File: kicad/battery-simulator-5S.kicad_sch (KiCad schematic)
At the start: 58 parts, among them J1 Conn_power_brd, J2 Conn_ctrl_brd, J7 Barrel_Jack, Q1 2N3904, Q2 NDP6020P, Q3 2SD2390, U1 LM324, U3 TL431LP, U4 LM317_TO-220

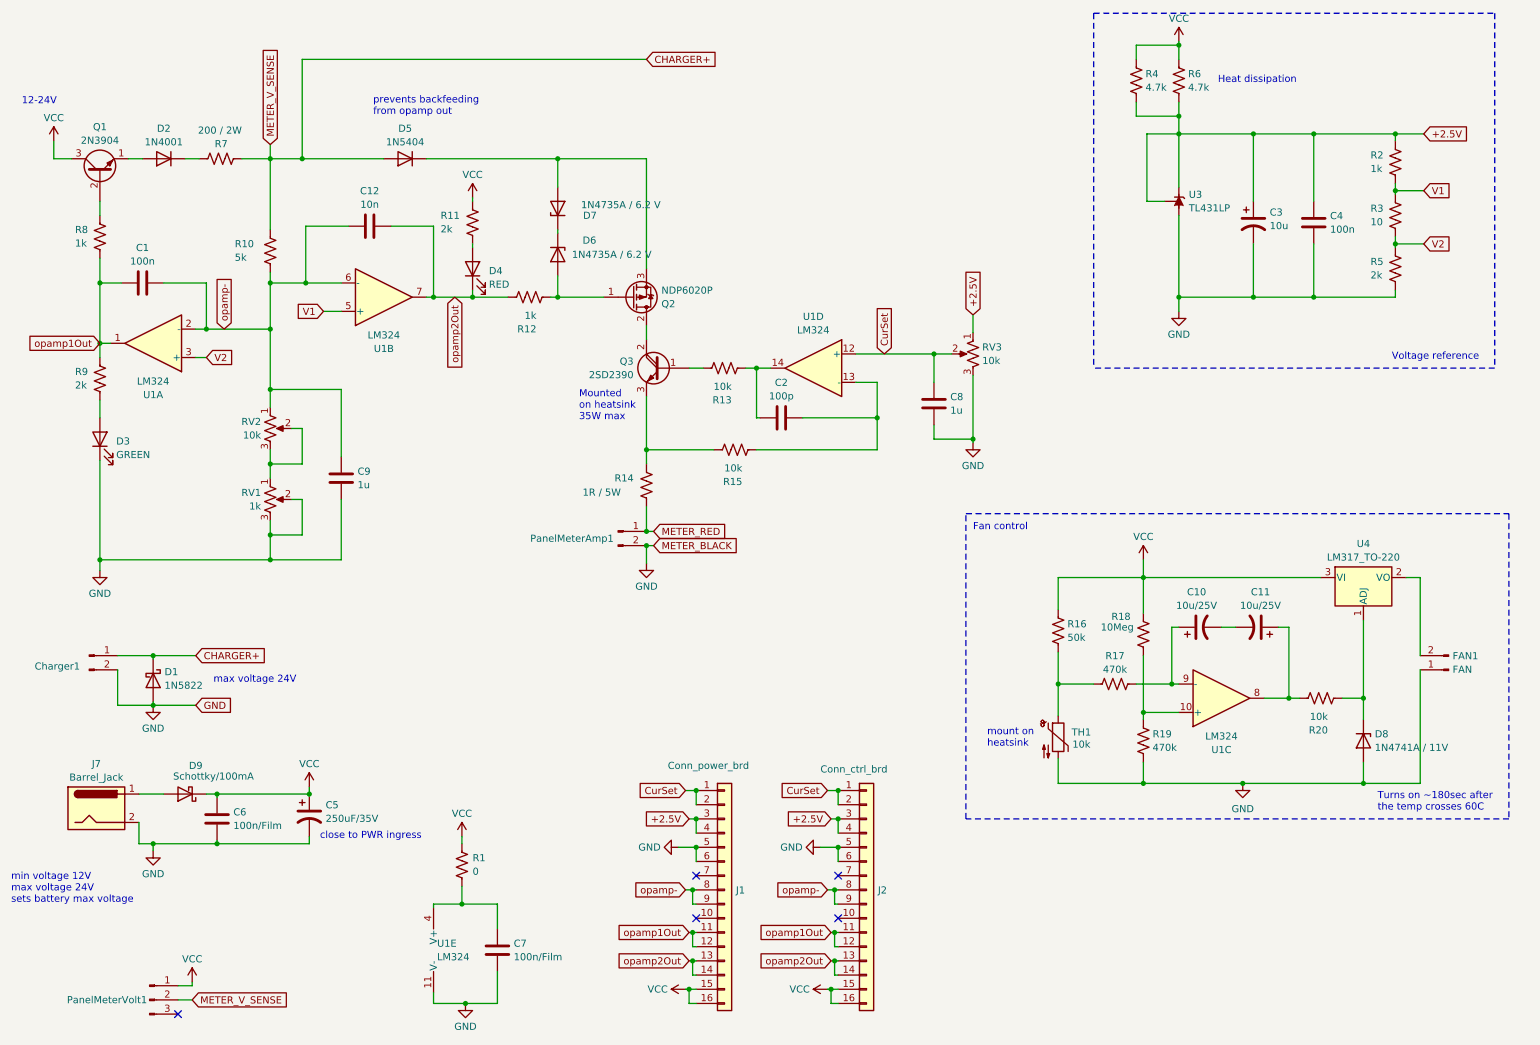
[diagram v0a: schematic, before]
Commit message: More ideas
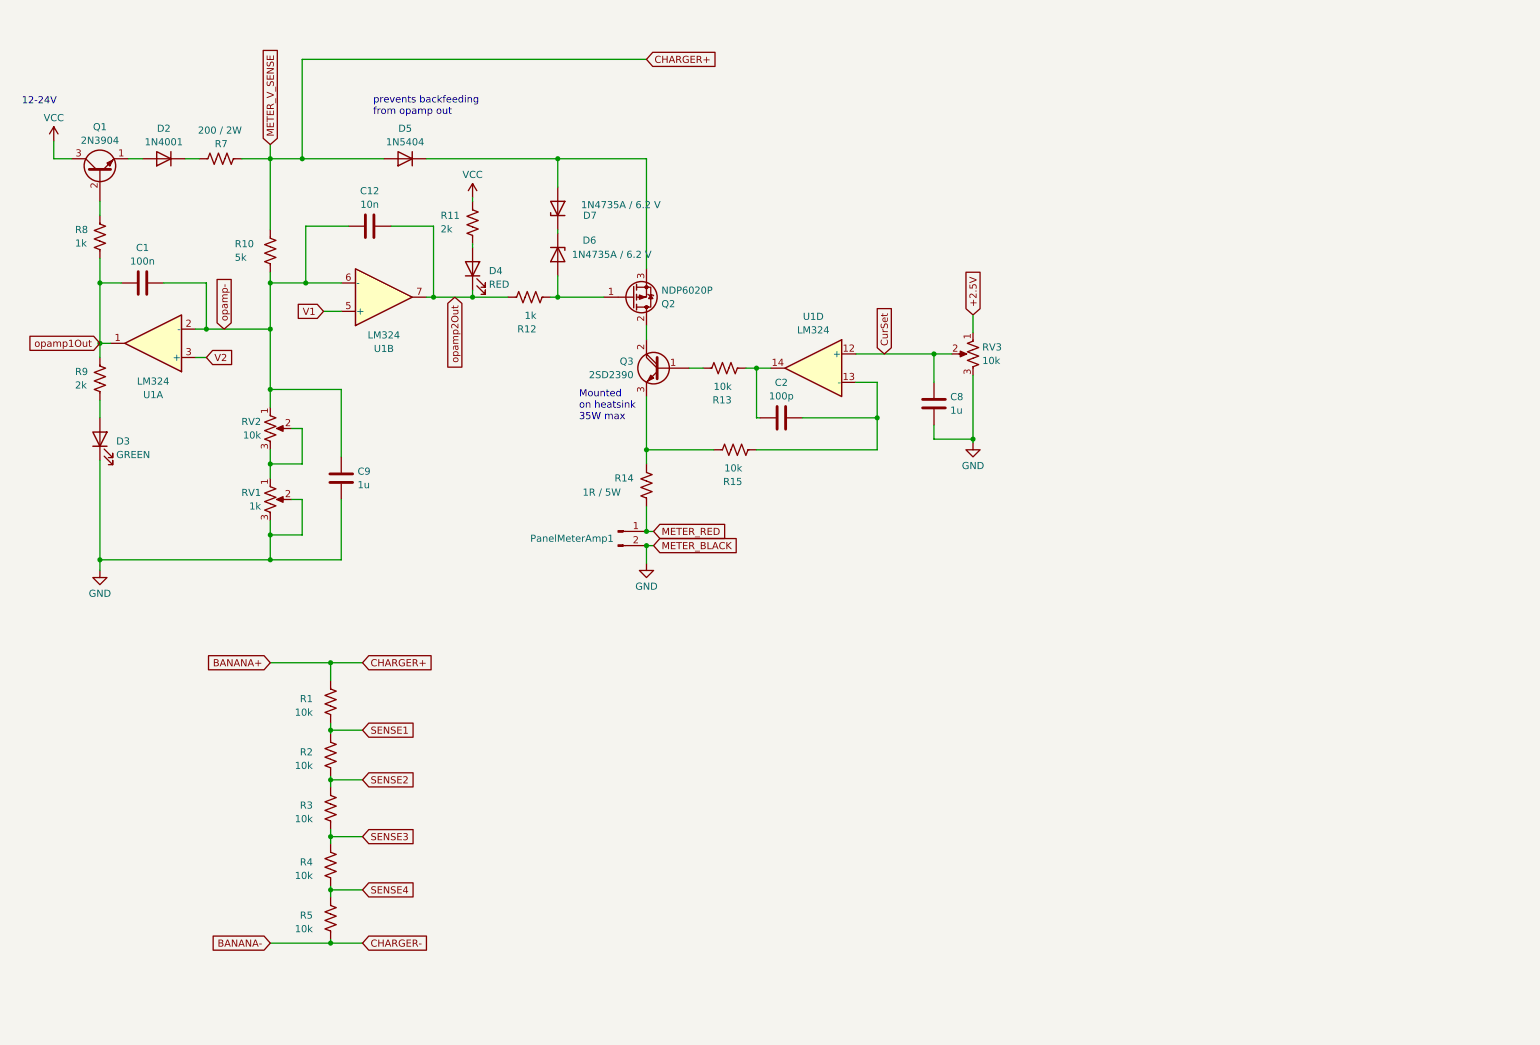
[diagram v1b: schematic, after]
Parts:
- removed C10, C11: 10u/25V, Capacitor_THT:CP_Radial_D5.0mm_P2.50mm, symbol Device:C_Polarized_US
- removed C3: 10u, Capacitor_THT:CP_Radial_D5.0mm_P2.50mm, symbol Device:C_Polarized_US
- removed C4: 100n, Capacitor_SMD:C_1206_3216Metric, symbol Device:C
- removed C5: 250uF/35V, Capacitor_THT:CP_Radial_D14.0mm_P5.00mm, symbol Device:C_Polarized_US
- removed C6, C7: 100n/Film, Capacitor_SMD:C_1206_3216Metric, symbol Device:C
- removed Charger1: Charger, Connector_Phoenix_MC_HighVoltage:PhoenixContact_MCV_1,5_2-G-5.08_1x02_P5.08mm_Vertical, symbol Connector:Conn_01x02_Pin
- removed D1: 1N5822, Diode_THT:D_DO-201AD_P5.08mm_Vertical_AnodeUp, symbol Diode:1N5822
- removed D8: 1N4741A / 11V, Diode_THT:D_DO-35_SOD27_P5.08mm_Vertical_KathodeUp, symbol Device:D_Zener
- removed D9: Schottky/100mA, Diode_SMD:D_SMA, symbol Device:D_Schottky
- removed FAN1: FAN, Connector_PinHeader_2.54mm:PinHeader_1x03_P2.54mm_Vertical, symbol Connector:Conn_01x02_Pin
- removed J1: Conn_power_brd, Connector_PinSocket_2.54mm:PinSocket_1x16_P2.54mm_Vertical, symbol Connector_Generic:Conn_01x16
- removed J2: Conn_ctrl_brd, Connector_PinHeader_2.54mm:PinHeader_1x16_P2.54mm_Horizontal, symbol Connector_Generic:Conn_01x16
- removed J7: Barrel_Jack, Connector_BarrelJack:BarrelJack_Horizontal, symbol Connector:Barrel_Jack
- removed PanelMeterVolt1: Panel Meter Volt, Connector_JST:JST_XH_B3B-XH-A_1x03_P2.50mm_Vertical, symbol Connector:Conn_01x03_Pin
- removed R16: 50k, Resistor_SMD:R_0805_2012Metric, symbol Device:R_US
- removed R17: 470k, Resistor_SMD:R_1206_3216Metric, symbol Device:R_US
- removed R18: 10Meg, Resistor_SMD:R_0805_2012Metric, symbol Device:R_US
- removed R19: 470k, Resistor_SMD:R_0805_2012Metric, symbol Device:R_US
- removed R20: 10k, Resistor_SMD:R_0805_2012Metric, symbol Device:R_US
- removed R6: 4.7k, Resistor_THT:R_Axial_DIN0207_L6.3mm_D2.5mm_P7.62mm_Horizontal, symbol Device:R_US
- removed TH1: 10k, Connector_JST:JST_XH_B2B-XH-A_1x02_P2.50mm_Vertical, symbol Device:Thermistor_NTC
- removed unit 3 of U1
- removed unit 5 of U1
- removed U3: TL431LP, Package_TO_SOT_THT:TO-92L_Wide, symbol Reference_Voltage:TL431LP
- removed U4: LM317_TO-220, Package_TO_SOT_THT:TO-220-3_Vertical, symbol Regulator_Linear:LM317_TO-220
- R1: value 0 -> 10k; footprint Resistor_SMD:R_1206_3216Metric -> Resistor_SMD:R_0805_2012Metric
- R2: value 1k -> 10k
- R3: value 10 -> 10k
- R4: value 4.7k -> 10k; footprint Resistor_THT:R_Axial_DIN0207_L6.3mm_D2.5mm_P7.62mm_Horizontal -> Resistor_SMD:R_0805_2012Metric
- R5: value 2k -> 10k
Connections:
- net CHARGER+ is gone; now on net BANANA+: D5.2 (A), R10.1, R7.2
- net +2.5V: no longer R2.1, R4.2
- net GND: no longer R5.2
- net V1: no longer R2.2, R3.1
- net V2: no longer R3.2, R5.1
- net VCC: no longer R1.1, R4.1
- net BANANA+: now reaches R1.2
- new net BANANA-: R5.1
- new net SENSE1: R1.1, R2.2
- new net SENSE2: R2.1, R3.2
- new net SENSE3: R3.1, R4.2
- new net SENSE4: R4.1, R5.2
- no-connect marks 5 -> 0
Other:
- note removed: "Fan control"
- note removed: "Heat dissipation"
- note removed: "Turns on ~180sec after the temp crosses 60C"
- note removed: "Voltage reference"
- note removed: "close to PWR ingress"
- note removed: "max voltage 24V"
- note removed: "min voltage 12V max voltage 24V sets battery max voltage"
- note removed: "mount on heatsink"
